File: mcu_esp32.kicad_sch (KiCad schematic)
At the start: 26 parts, among them SW2 IO0, SW3 IO0, T1 S8050, T2 S8050, U5 CP2102N-Axx-xQFN28, U6 ESP32-WROOM-32D

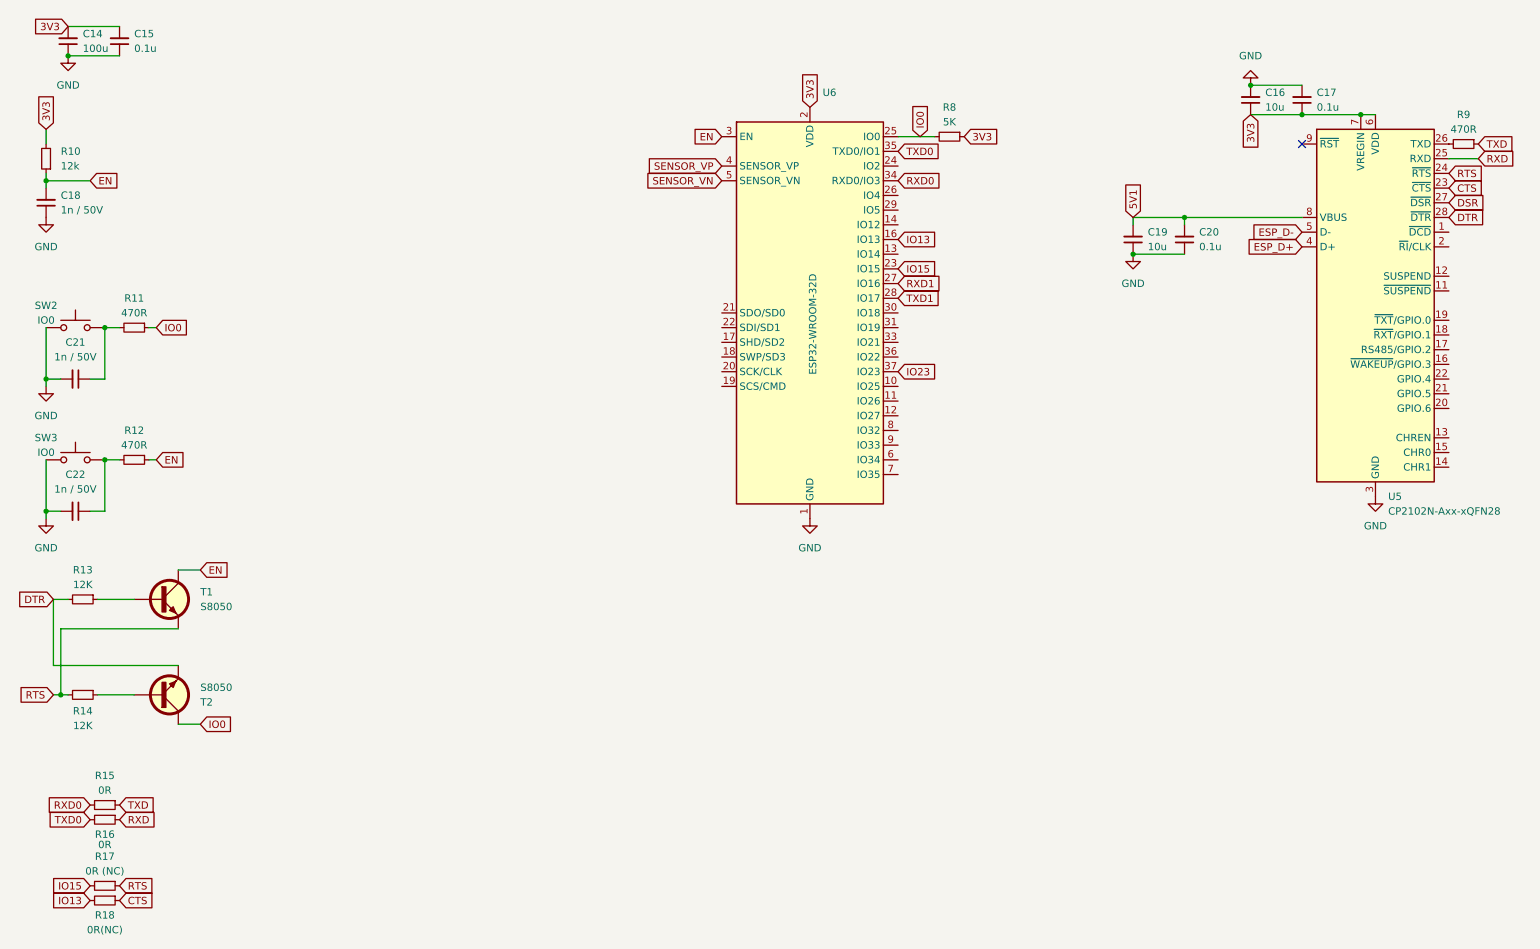
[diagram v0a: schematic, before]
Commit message: Visual Improvements
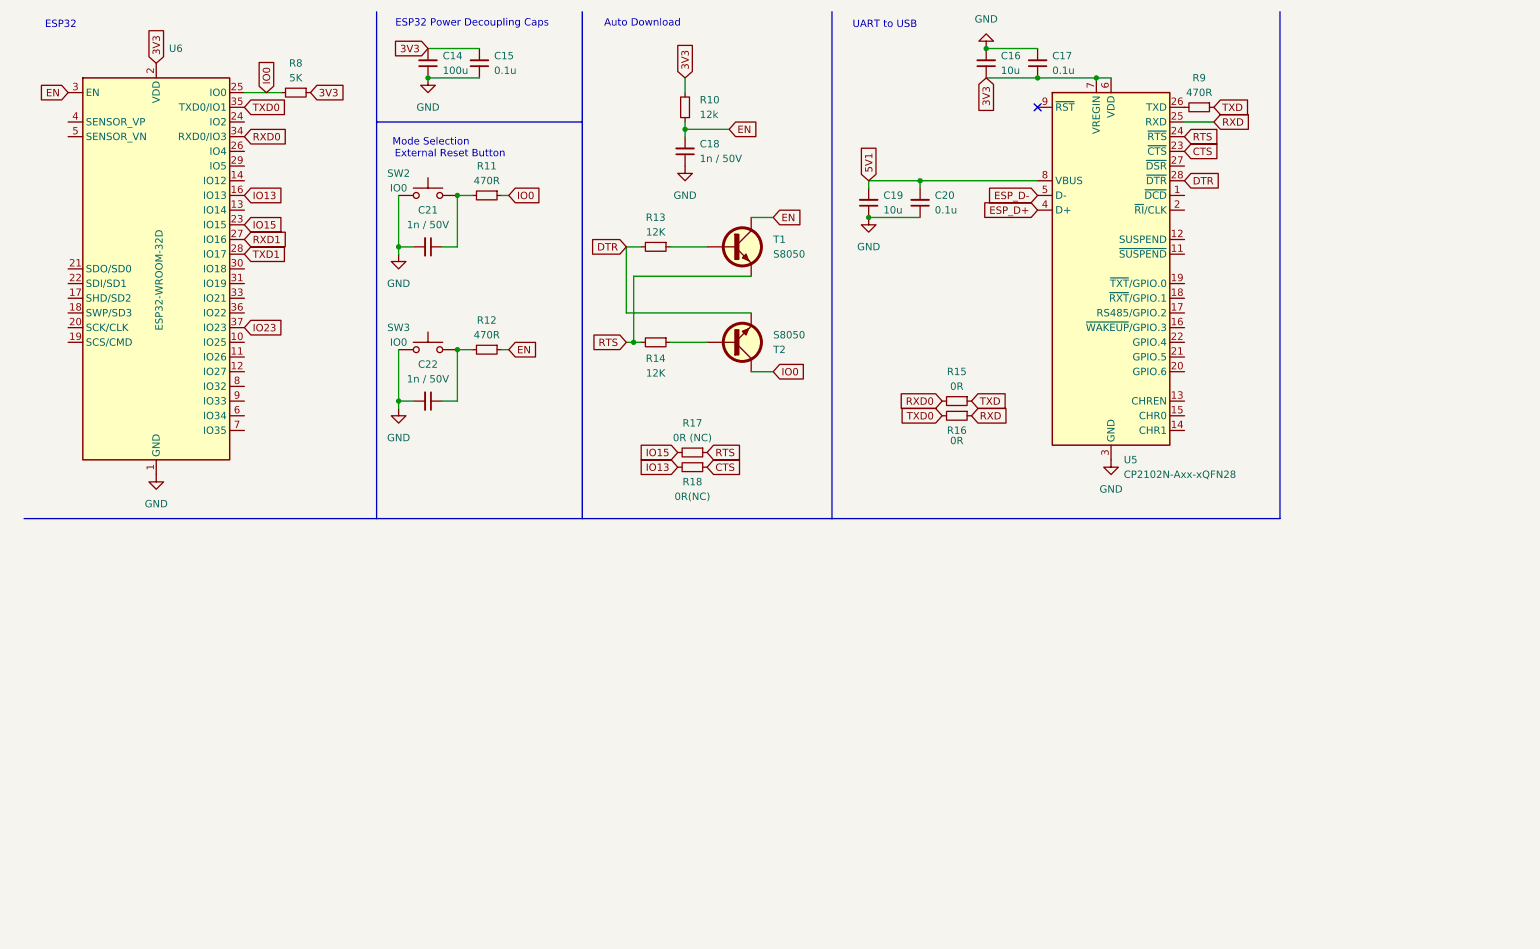
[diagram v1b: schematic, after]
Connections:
- net DSR: no longer names the net of U5.27 (~{DSR})
- net SENSOR_VN: no longer names the net of U6.5 (SENSOR_VN)
- net SENSOR_VP: no longer names the net of U6.4 (SENSOR_VP)
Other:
- note added: "Auto Download"
- note added: "ESP32"
- note added: "ESP32 Power Decoupling Caps"
- note added: "External Reset Button"
- note added: "Mode Selection"
- note added: "UART to USB"
- moved on the sheet: C14, C15, C16, C17, C18, C19, C20, C21, C22, R10, R11, R12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
